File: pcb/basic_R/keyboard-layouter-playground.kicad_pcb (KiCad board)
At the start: 2 copper layers, 243 x 151.8 mm, 129 parts, among them J2 MJ-4PP-9, SW103 SW_Push, SW104 SW_Push, SW105 SW_Push, SW202 SW_Push, SW303 SW_Push, SW305 SW_Push, SW31 SW_Push, SW32 SW_Push, SW33 SW_Push, SW34 SW_Push, SW35 SW_Push, SW36 SW_Push, SW37 SW_Push, SW38 SW_Push, SW39 SW_Push, SW40 SW_Push, SW41 SW_Push, SW42 SW_Push, SW43 SW_Push, SW44 SW_Push, SW45 SW_Push, SW46 SW_Push, SW47 SW_Push, SW48 SW_Push, SW49 SW_Push, SW50 SW_Push, SW51 SW_Push, SW52 SW_Push, SW53 SW_Push, SW54 SW_Push, SW55 SW_Push, SW56 SW_Push, SW57 SW_Push, SW58 SW_Push, SW59 SW_Push, SW60 SW_Push, SW61 SW_Push, SW62 SW_Push, SW63 SW_Push, SW64 SW_Push, SW65 SW_Push, SW66 SW_Push, SW67 SW_Push, SW68 SW_Push, SW69 SW_Push, SW70 SW_Push, SW71 SW_Push, SW72 SW_Push, SW73 SW_Push, SW74 SW_Push, SW75 SW_Push, SW76 SW_Push, SW77 SW_Push, SW78 SW_Push, SW79 SW_Push, SW80 SW_Push, SW81 SW_Push, SW82 SW_Push, SW83 SW_Push, SW84 SW_Push, SW85 SW_Push, SW901 SW_Push, U2 Elite-C

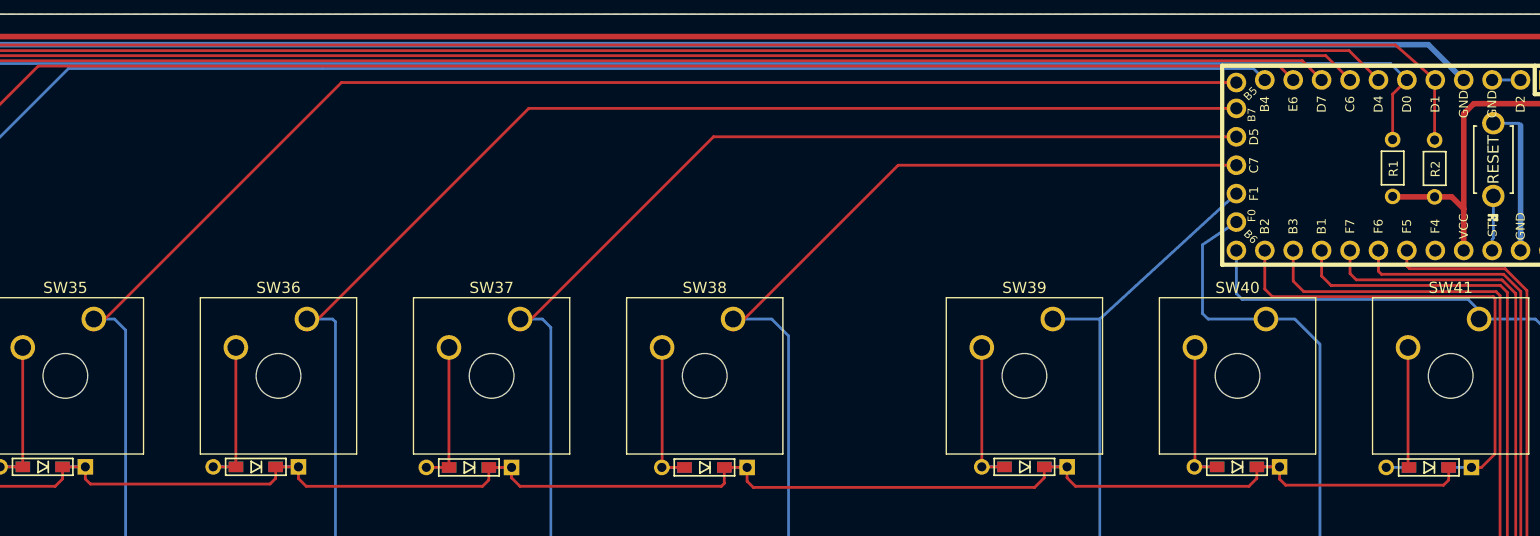
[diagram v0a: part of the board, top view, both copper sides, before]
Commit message: case data make
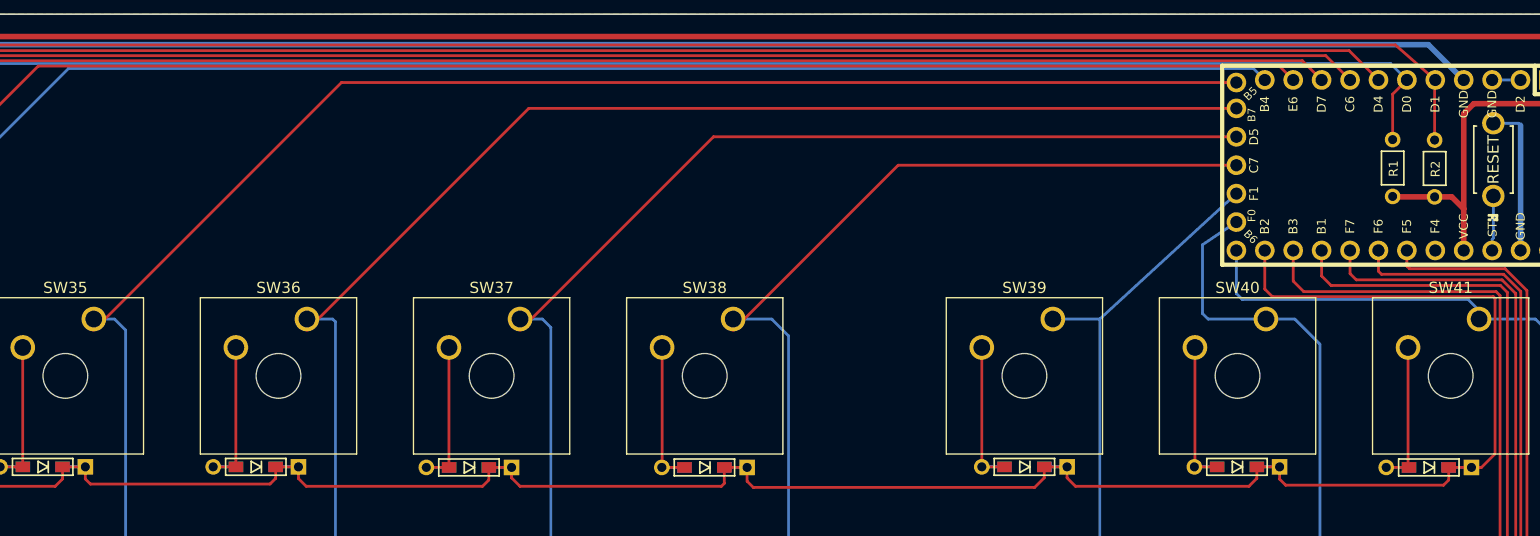
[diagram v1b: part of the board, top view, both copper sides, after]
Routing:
- net row7: track 298.1 -> 300.1 mm
- net Net-(D41-Pad1): track 12.8 -> 14.8 mm
